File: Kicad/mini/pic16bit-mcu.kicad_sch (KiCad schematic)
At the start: 32 parts, among them K201 *Power & UART, K202 MCU 1, K203 MCU 1, K204 ICSP, K205 MCU 2, K206 MCU 2, U201 TLV1117-33, U202 PIC24/dsPIC32

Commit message: Up
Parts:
- K201: symbol tronixio:FCI-USB-TYPE-B-MICRO-THT -> tronixio:FCI-USB-TYPE-B-MICRO-TH
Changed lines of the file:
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@@
     )
   )
-  (symbol (lib_id "tronixio:FCI-USB-TYPE-B-MICRO-THT") (at 38.1 175.26 0) (unit 1)
+  (symbol (lib_id "tronixio:FCI-USB-TYPE-B-MICRO-TH") (at 38.1 175.26 0) (unit 1)
     (in_bom yes) (on_board yes) (dnp no)
     (property "Reference" "K201" (at 38.1 162.56 0)

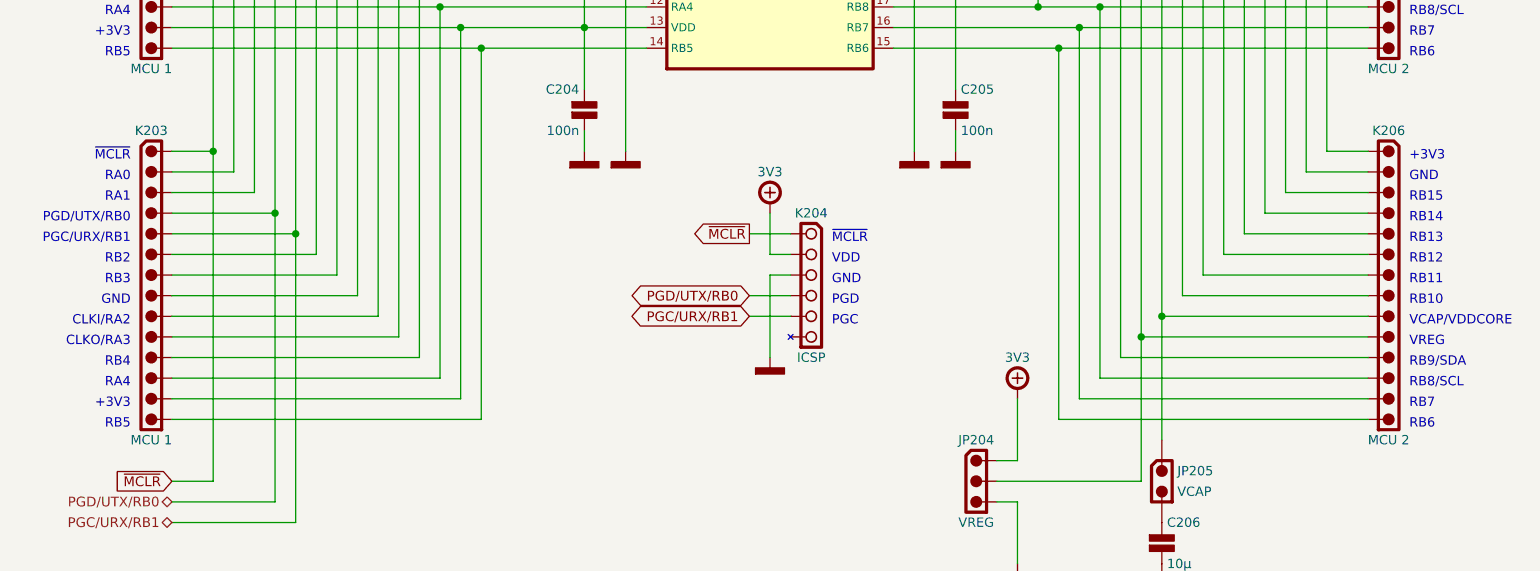
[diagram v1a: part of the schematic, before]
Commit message: Up
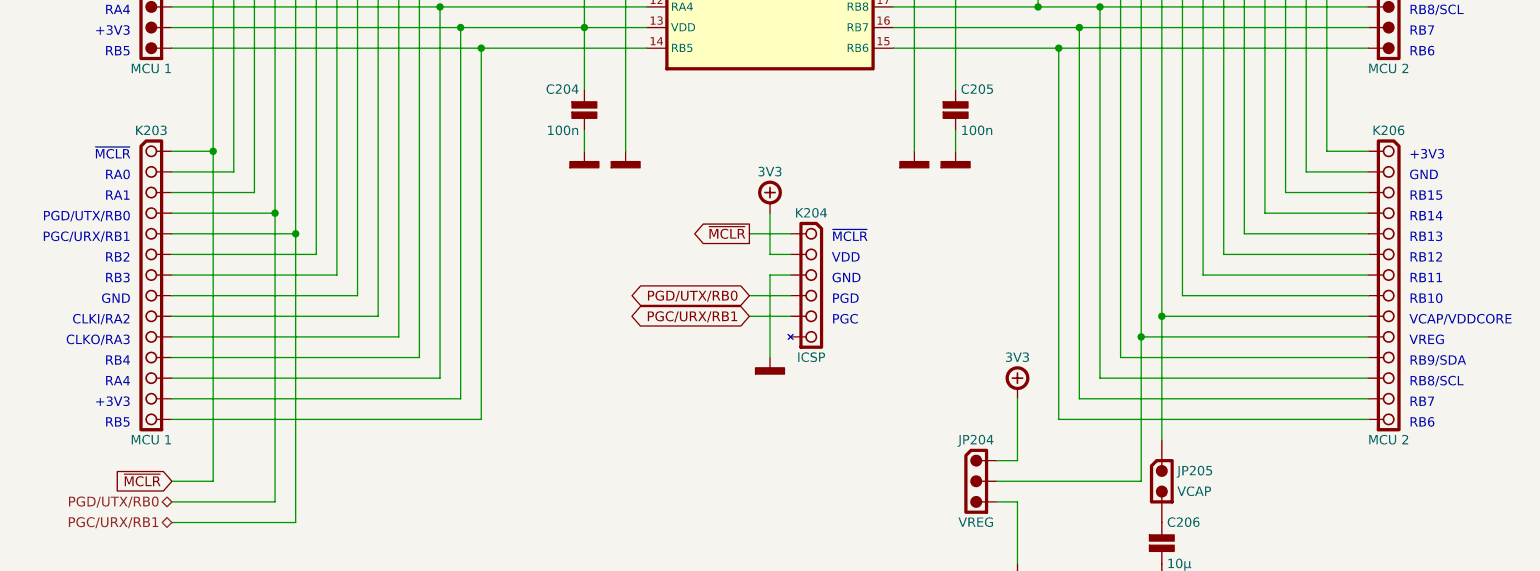
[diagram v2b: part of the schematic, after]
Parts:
- K204: symbol tronixio:MICROCHIP-ICSP-F-1X06 -> tronixio:MICROCHIP-ICSP-F-RIGHT-ANGLE-TH
- U202: footprint tronixio:DIP-28-W762-SOCKET -> tronixio:DIP-28-W762
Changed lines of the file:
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@@
       (effects (font (size 1.15 1.15)) (justify right))
     )
-    (property "Footprint" "tronixio:DIP-28-W762-SOCKET" (at 144.78 96.52 0) (do_not_autoplace)
+    (property "Footprint" "tronixio:DIP-28-W762" (at 144.78 96.52 0) (do_not_autoplace)
       (effects (font (size 1 1)) hide)
     )
@@
     )
   )
-  (symbol (lib_id "tronixio:MICROCHIP-ICSP-F-1X06") (at 149.86 111.76 0) (unit 1)
+  (symbol (lib_id "tronixio:MICROCHIP-ICSP-F-RIGHT-ANGLE-TH") (at 149.86 111.76 0) (unit 1)
     (in_bom yes) (on_board yes) (dnp no)
     (property "Reference" "K204" (at 149.86 109.22 0)

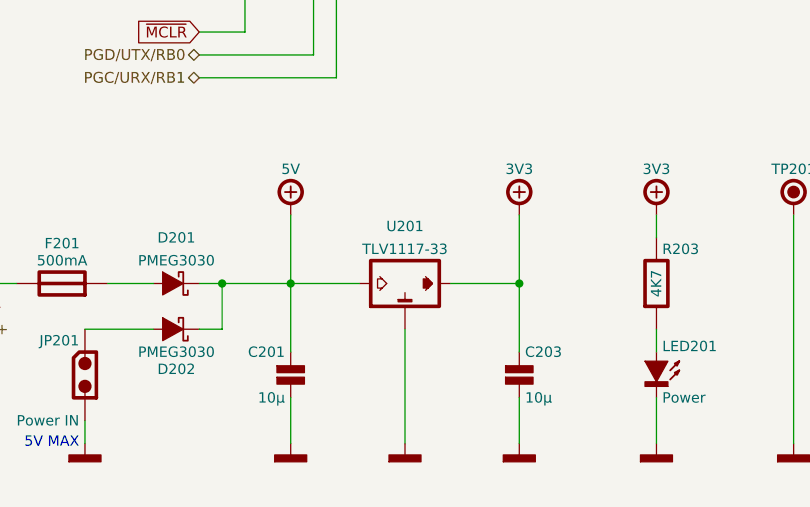
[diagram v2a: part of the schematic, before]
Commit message: Update
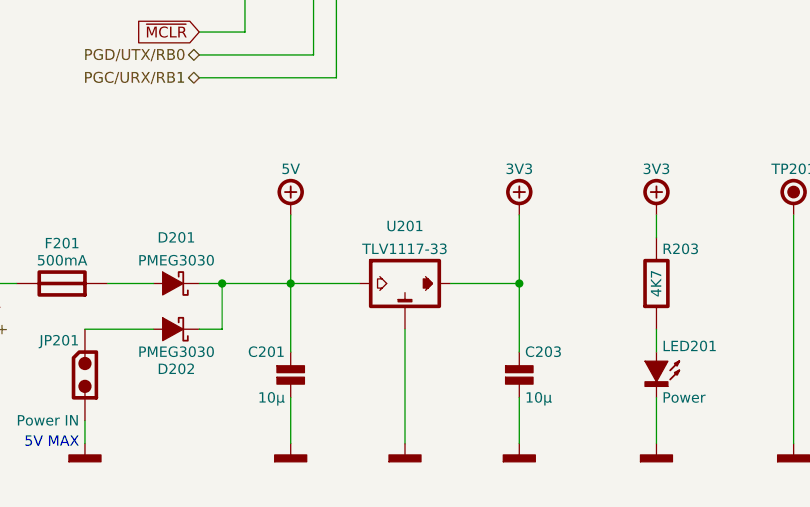
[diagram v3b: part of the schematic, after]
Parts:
- C201, C203, C206: Mouser 791-1206X106J250CT -> 80-C1206C106J3R
- D201, D202: symbol tronixio:NEXPERIA-PMEG3030 -> tronixio:NEXPERIA-PMEG3030-SOD
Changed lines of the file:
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@@
       (effects (font (size 1.15 1.15)) (justify left) hide)
     )
-    (property "Mouser" "791-1206X106J250CT" (at 193.04 162.56 0) (do_not_autoplace)
+    (property "Mouser" "80-C1206C106J3R" (at 193.04 162.56 0) (do_not_autoplace)
       (effects (font (size 1 1)) hide)
     )
@@
     )
   )
-  (symbol (lib_id "tronixio:NEXPERIA-PMEG3030") (at 68.58 175.26 180) (unit 1)
+  (symbol (lib_id "tronixio:NEXPERIA-PMEG3030-SOD") (at 68.58 175.26 180) (unit 1)
     (in_bom yes) (on_board yes) (dnp no)
     (property "Reference" "D202" (at 68.58 179.705 0)
@@
       (effects (font (size 1.15 1.15)) (justify left) hide)
     )
-    (property "Mouser" "791-1206X106J250CT" (at 81.28 193.04 0) (do_not_autoplace)
+    (property "Mouser" "80-C1206C106J3R" (at 81.28 193.04 0) (do_not_autoplace)
       (effects (font (size 1 1)) hide)
     )
@@
       (effects (font (size 1.15 1.15)) (justify left) hide)
     )
-    (property "Mouser" "791-1206X106J250CT" (at 106.68 193.04 0) (do_not_autoplace)
+    (property "Mouser" "80-C1206C106J3R" (at 106.68 193.04 0) (do_not_autoplace)
       (effects (font (size 1 1)) hide)
     )
@@
     )
   )
-  (symbol (lib_id "tronixio:NEXPERIA-PMEG3030") (at 68.58 170.18 180) (unit 1)
+  (symbol (lib_id "tronixio:NEXPERIA-PMEG3030-SOD") (at 68.58 170.18 180) (unit 1)
     (in_bom yes) (on_board yes) (dnp no)
     (property "Reference" "D201" (at 68.58 165.1 0)

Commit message: Update Mini Kicad 8
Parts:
- U201: footprint tronixio:SOT-223-3 -> tronixio:SOT-223-3-TABPIN2
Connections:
- net +3V3 renamed POWER-+3V3
- net +5V renamed POWER-+5V
- net GND renamed POWER-GND
